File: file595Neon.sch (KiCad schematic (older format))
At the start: 33 parts, among them U1 74HC595

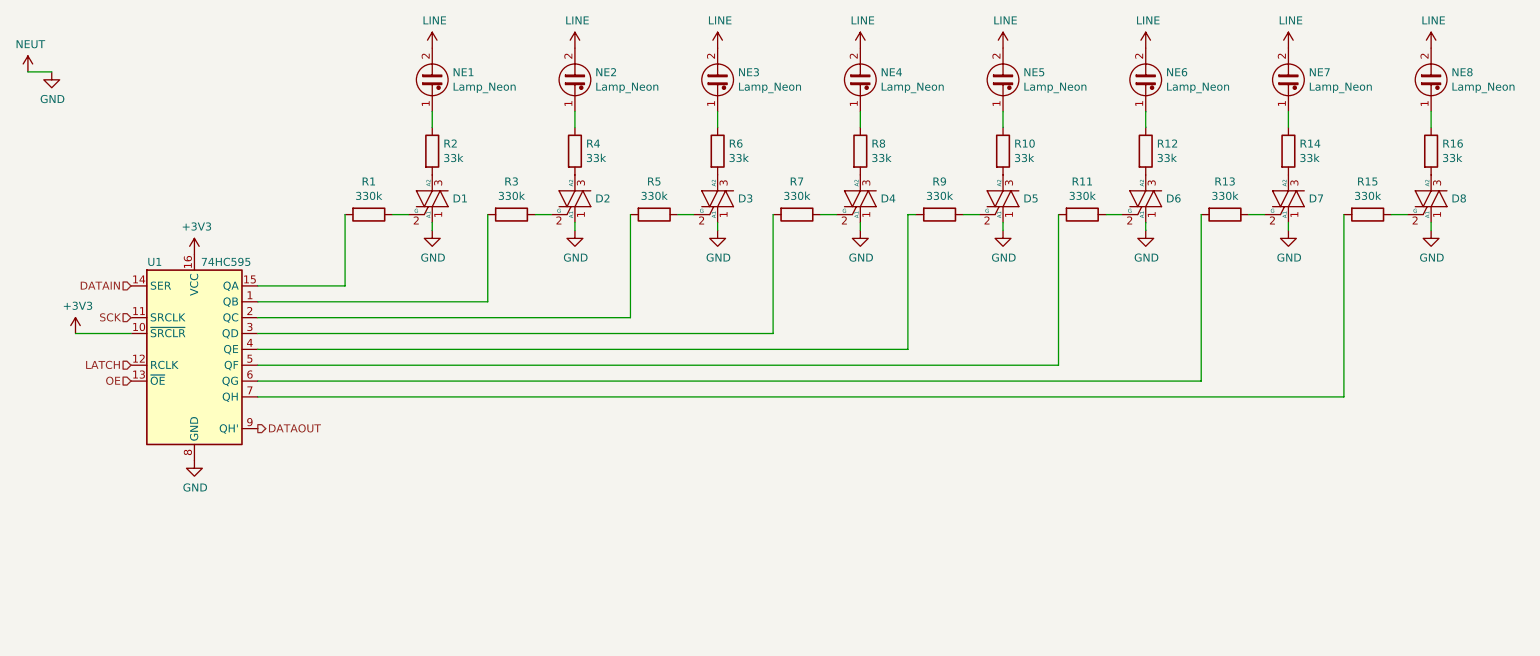
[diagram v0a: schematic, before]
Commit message: First row
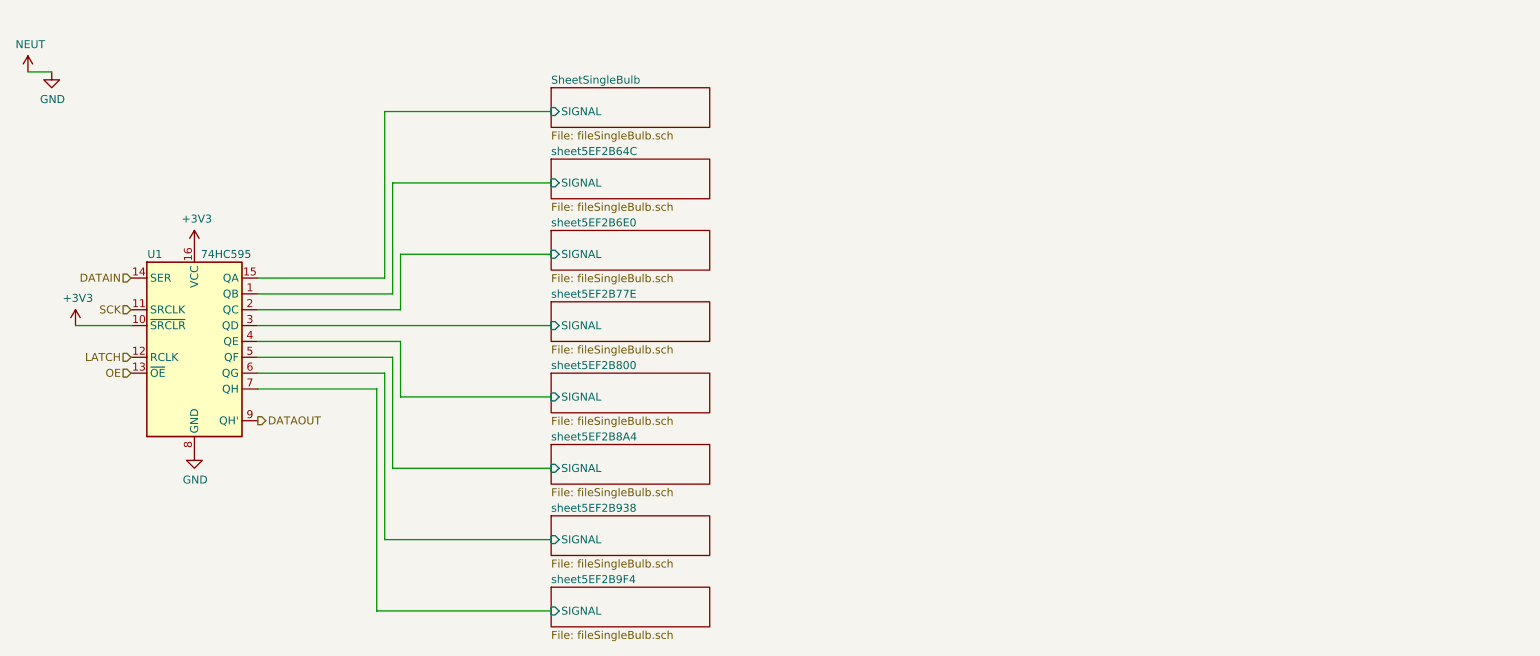
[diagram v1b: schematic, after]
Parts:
- removed D1, D2, D3, D4, D5, D6, D7, D8: Q_TRIAC_A1GA2, Package_TO_SOT_SMD:SOT-23, symbol Device:Q_TRIAC_A1GA2
- removed NE1, NE2, NE3, NE4, NE5, NE6, NE7, NE8: Lamp_Neon, Connector_PinHeader_2.54mm:PinHeader_1x02_P2.54mm_Horizontal, symbol Device:Lamp_Neon
- removed R1, R11, R13, R15, R3, R5, R7, R9: 330k, Resistor_SMD:R_0402_1005Metric, symbol Device:R
- removed R10, R12, R14, R16, R2, R4, R6, R8: 33k, Resistor_SMD:R_0603_1608Metric, symbol Device:R
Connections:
- net sheet5EF2B64C/SIGNAL: now reaches U1.1 (QB)
- net SheetSingleBulb/SIGNAL: now reaches U1.15 (QA)
- net sheet5EF2B6E0/SIGNAL: now reaches U1.2 (QC)
- net sheet5EF2B77E/SIGNAL: now reaches U1.3 (QD)
- net sheet5EF2B800/SIGNAL: now reaches U1.4 (QE)
- net sheet5EF2B8A4/SIGNAL: now reaches U1.5 (QF)
- net sheet5EF2B938/SIGNAL: now reaches U1.6 (QG)
- net sheet5EF2B9F4/SIGNAL: now reaches U1.7 (QH)
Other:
- moved on the sheet: U1
